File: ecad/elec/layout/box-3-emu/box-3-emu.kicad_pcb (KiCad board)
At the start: 2 copper layers, 72.5 x 63.9 mm, 71 parts

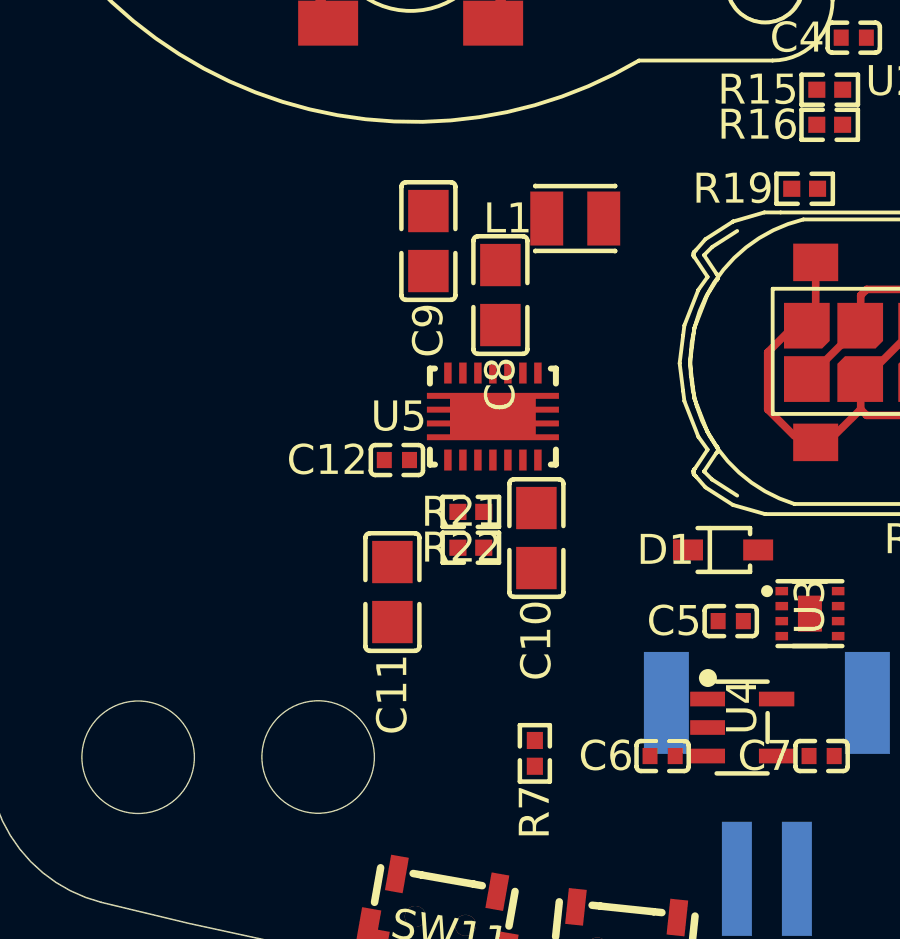
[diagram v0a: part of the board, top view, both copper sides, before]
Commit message: further layout changes
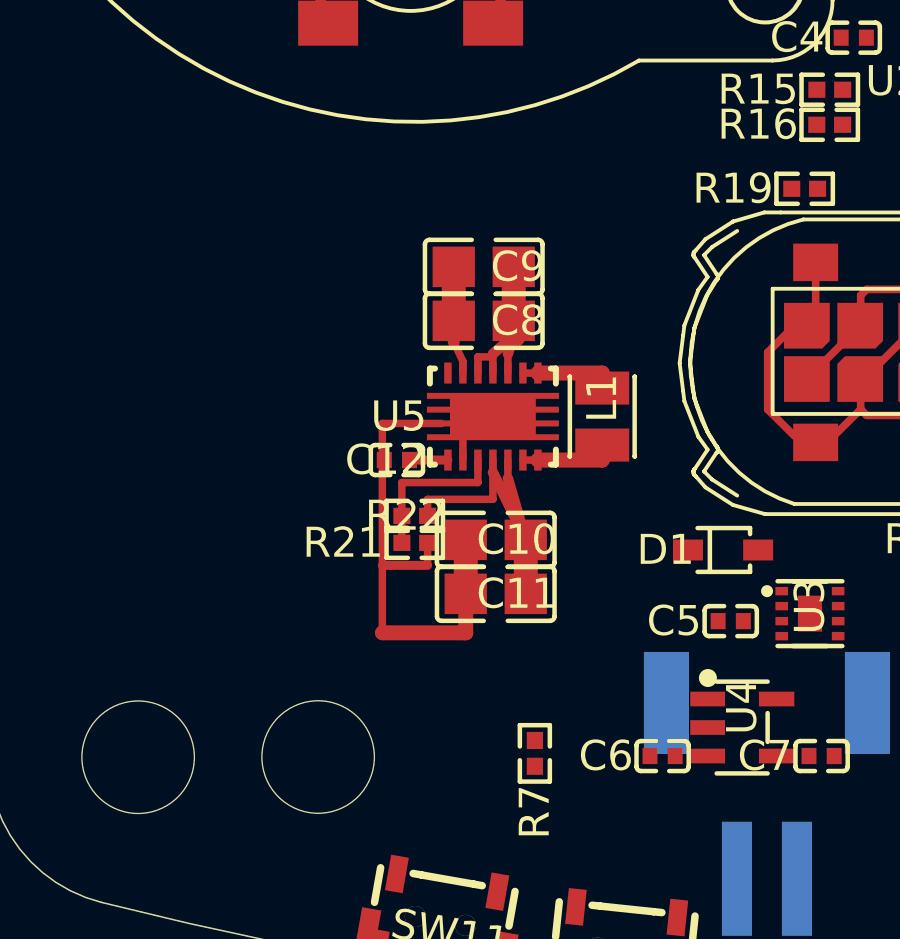
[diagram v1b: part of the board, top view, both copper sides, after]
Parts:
- moved L1 6.66 mm to (134.8, 125.5), turned to 270 degrees
- moved C11 3.45 mm to (131.3, 131.4), turned to 180 degrees
- moved R22 2.15 mm to (128.6, 128.8)
- moved R21 2.14 mm to (128.6, 129.7), turned to 0 degrees
- moved C9 2.04 mm to (130.9, 120.5), turned to 180 degrees
- moved C10 1.36 mm to (131.3, 129.6), turned to 180 degrees
- moved C8 1.02 mm to (130.9, 122.3), turned to 180 degrees
- turned C12 to 180 degrees
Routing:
- net gnd: track 0.00 -> 21.5 mm
- net vcc_5v: track 0.00 -> 11.1 mm
- net vbat: track 0.00 -> 7.45 mm
- net FB: track 0.00 -> 5.30 mm
- net 2: track 0.00 -> 3.15 mm
- net 1: track 0.00 -> 3.15 mm
